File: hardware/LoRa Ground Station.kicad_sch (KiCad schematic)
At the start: 51 parts, among them J1 RFPC-SMA28-F, J2 USB_C_Receptacle_USB2.0_14P, SW1 BOOT, SW2 RESET, U1 RP2040, U2 SX1262IMLTRT, U3 PE4259, U4 AP2112K-3.3, U5 W25Q128JVS, Y1 ECS-TXO-25CSMV-320-DY-TR, Y2 ABM8G-12.000MHZ-18-D2Y-T

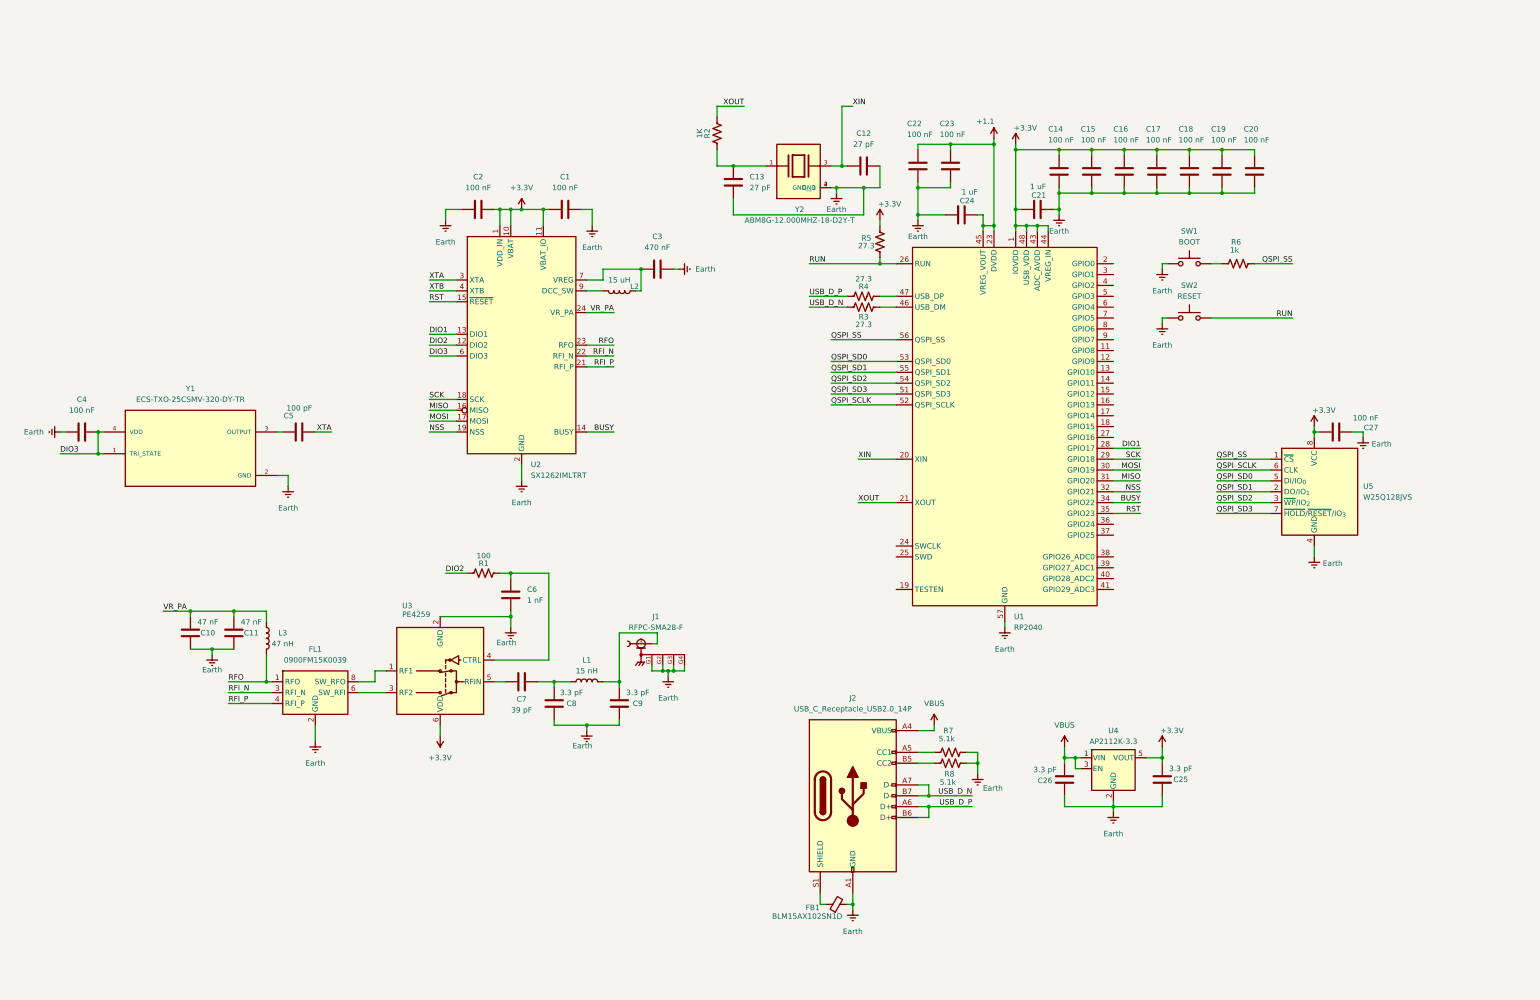
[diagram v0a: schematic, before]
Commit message: Add files via upload
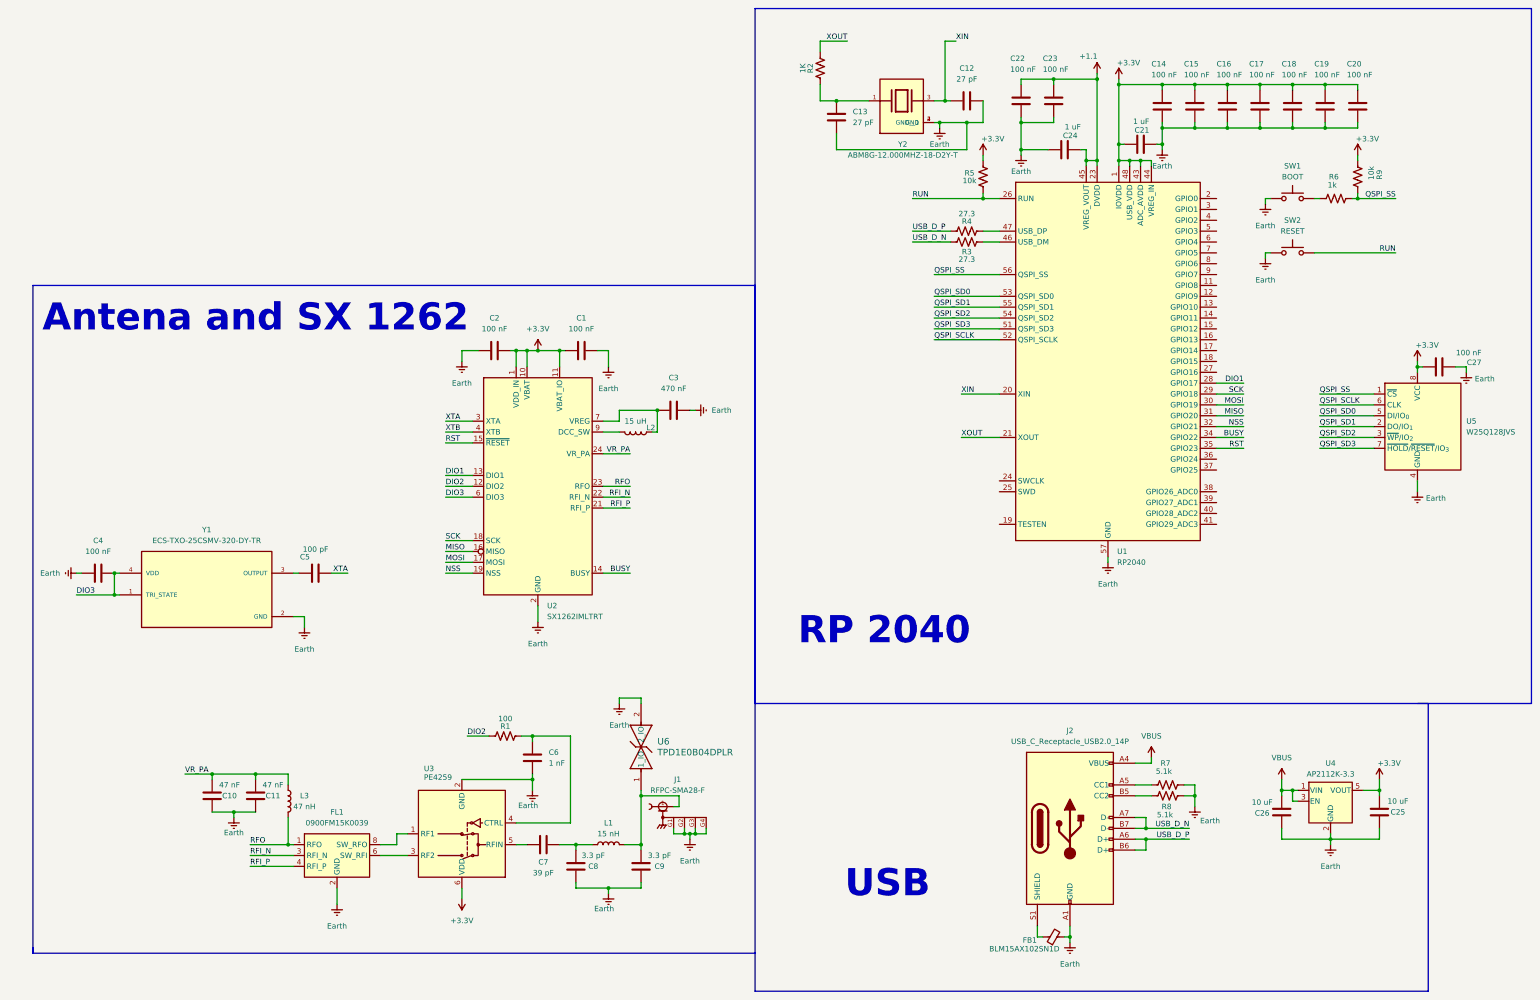
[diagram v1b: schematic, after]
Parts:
- added R9: 10k, Resistor_SMD:R_0402_1005Metric, symbol Device:R_US
- added U6: TPD1E0B04DPLR, footprints3:DPL0002A-MFG, symbol 2026-05-31_05-08-26:TPD1E0B04DPLR
- C25, C26: value 3.3 pF -> 10 uF; footprint Capacitor_SMD:C_0402_1005Metric -> Capacitor_SMD:C_0603_1608Metric
- R5: value 27.3 -> 10k
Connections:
- net +3.3V: now also R9.1
- net Earth: now also U6.2 (2_IO)
- net QSPI_SS: now also R9.2
- net at C9.2, J1.1, L1.2: now also U6.1 (1_IO)
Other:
- note added: "Antena and SX 1262"
- note added: "RP 2040"
- note added: "USB"
- moved on the sheet: C1, C10, C11, C12, C13, C14, C15, C16, C17, C18, C19, C2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
